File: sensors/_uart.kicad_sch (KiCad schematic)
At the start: 22 parts, among them J5 JP_GPS, J6 JP_RADIO, U1 SC16IS752IPW, Y1 14.7456MHz

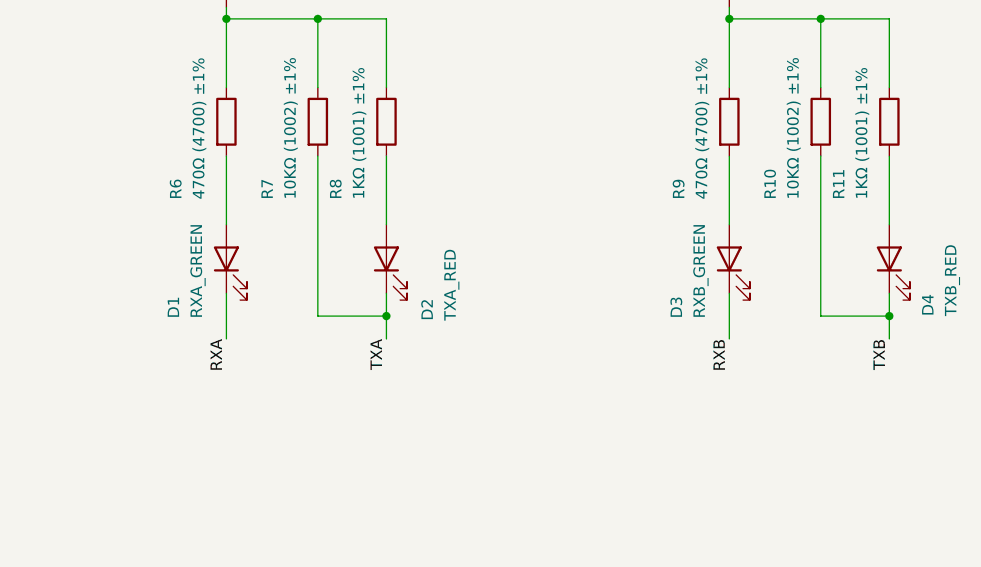
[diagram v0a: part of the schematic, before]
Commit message: routing
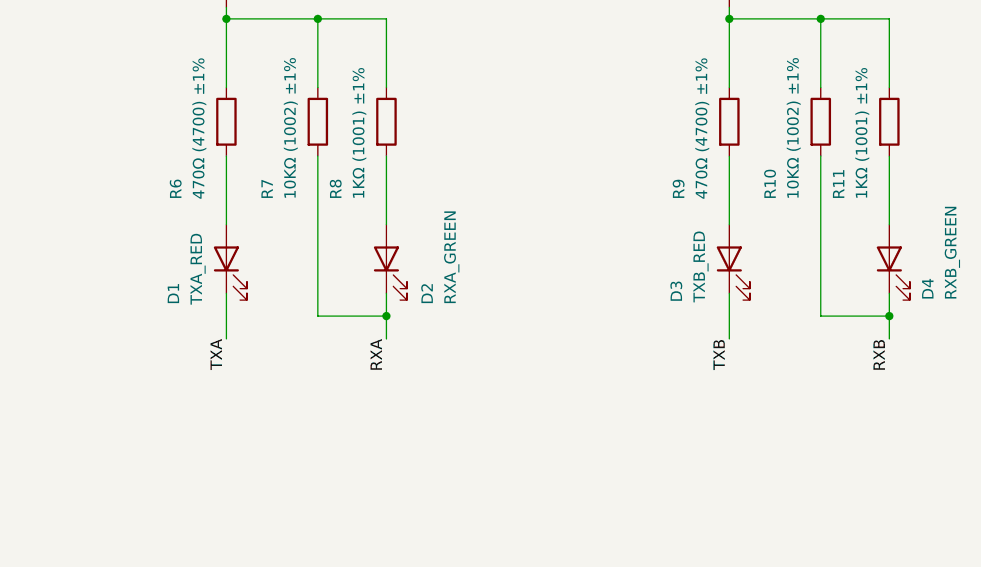
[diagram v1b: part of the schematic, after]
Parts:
- D1: value RXA_GREEN -> TXA_RED
- D2: value TXA_RED -> RXA_GREEN
- D3: value RXB_GREEN -> TXB_RED
- D4: value TXB_RED -> RXB_GREEN
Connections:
- net RXA: now also D2.1 (K), R7.2; no longer D1.1 (K)
- net RXB: now also D4.1 (K), R10.2; no longer D3.1 (K)
- net TXA: now also D1.1 (K); no longer D2.1 (K), R7.2
- net TXB: now also D3.1 (K); no longer D4.1 (K), R10.2
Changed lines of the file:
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@@
 	)
 	(label "RXA"
-		(at 271.78 105.41 270)
+		(at 289.56 105.41 270)
 		(effects
 			(font
@@
 	)
 	(label "RXB"
-		(at 327.66 105.41 270)
+		(at 345.44 105.41 270)
 		(effects
 			(font
@@
 	)
 	(label "TXB"
-		(at 345.44 105.41 270)
+		(at 327.66 105.41 270)
 		(effects
 			(font
@@
 	)
 	(label "TXA"
-		(at 289.56 105.41 270)
+		(at 271.78 105.41 270)
 		(effects
 			(font
@@
 		(dnp no)
 		(property "Reference" "D3"
-			(at 321.818 103.124 0)
+			(at 321.818 101.346 0)
 			(show_name no)
 			(do_not_autoplace no)
@@
 			)
 		)
-		(property "Value" "RXB_GREEN"
-			(at 324.358 103.124 0)
+		(property "Value" "TXB_RED"
+			(at 324.358 101.346 0)
 			(show_name no)
 			(do_not_autoplace no)
@@
 		(dnp no)
 		(property "Reference" "D1"
-			(at 265.938 103.124 0)
+			(at 265.938 101.6 0)
 			(show_name no)
 			(do_not_autoplace no)
@@
 			)
 		)
-		(property "Value" "RXA_GREEN"
-			(at 268.478 103.124 0)
+		(property "Value" "TXA_RED"
+			(at 268.478 101.6 0)
 			(show_name no)
 			(do_not_autoplace no)
@@
 		(dnp no)
 		(property "Reference" "D4"
-			(at 349.758 102.87 0)
+			(at 349.758 101.092 0)
 			(show_name no)
 			(do_not_autoplace no)
@@
 			)
 		)
-		(property "Value" "TXB_RED"
-			(at 352.298 102.87 0)
+		(property "Value" "RXB_GREEN"
+			(at 352.298 101.092 0)
 			(show_name no)
 			(do_not_autoplace no)
@@
 		(dnp no)
 		(property "Reference" "D2"
-			(at 294.132 103.378 0)
+			(at 294.132 101.6 0)
 			(show_name no)
 			(do_not_autoplace no)
@@
 			)
 		)
-		(property "Value" "TXA_RED"
-			(at 296.672 103.378 0)
-			(show_name no)
-			(do_not_autoplace no)
+		(property "Value" "RXA_GREEN"
+			(at 296.672 101.6 0)
+			(show_name no)
+			(do_not_autoplace no)
